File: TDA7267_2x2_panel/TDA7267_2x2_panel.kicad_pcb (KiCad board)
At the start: 2 copper layers, 90 x 84 mm, 72 parts, among them U1 TDA7267

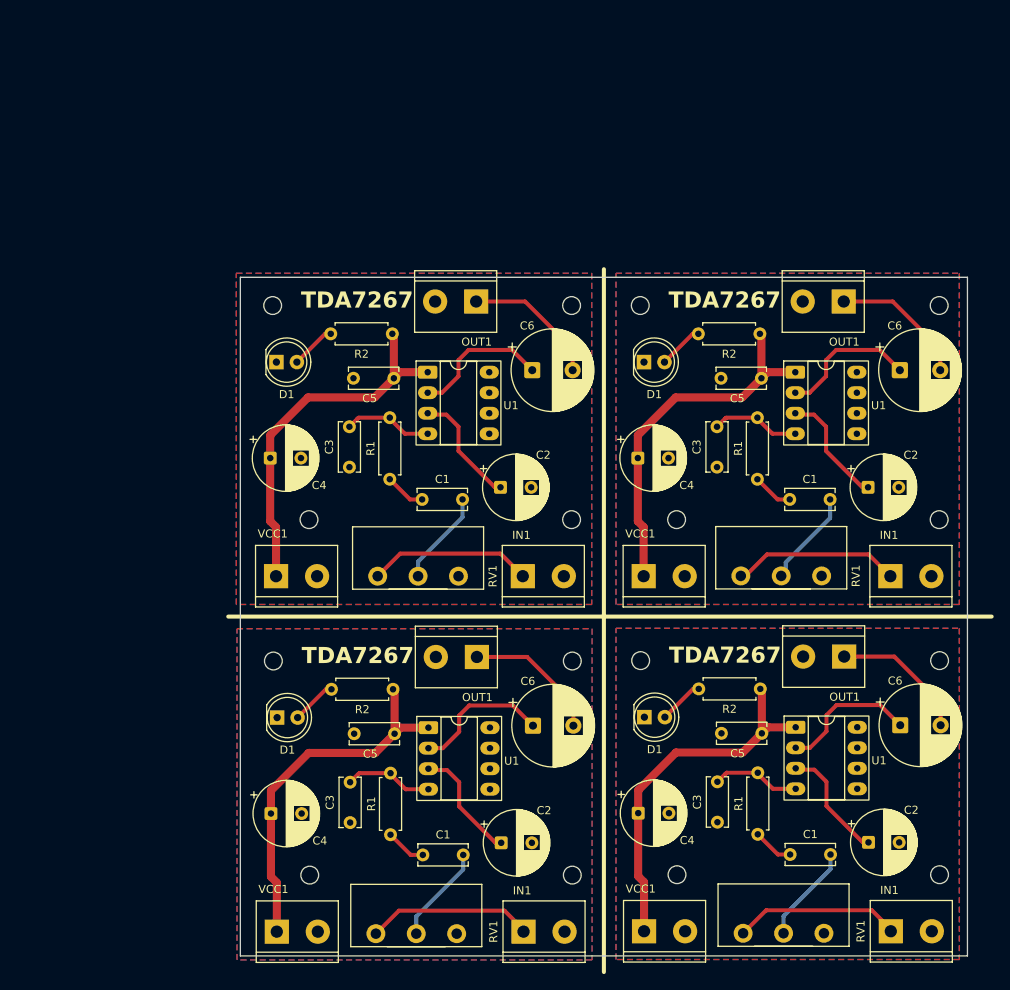
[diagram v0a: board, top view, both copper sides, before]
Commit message: Improvements
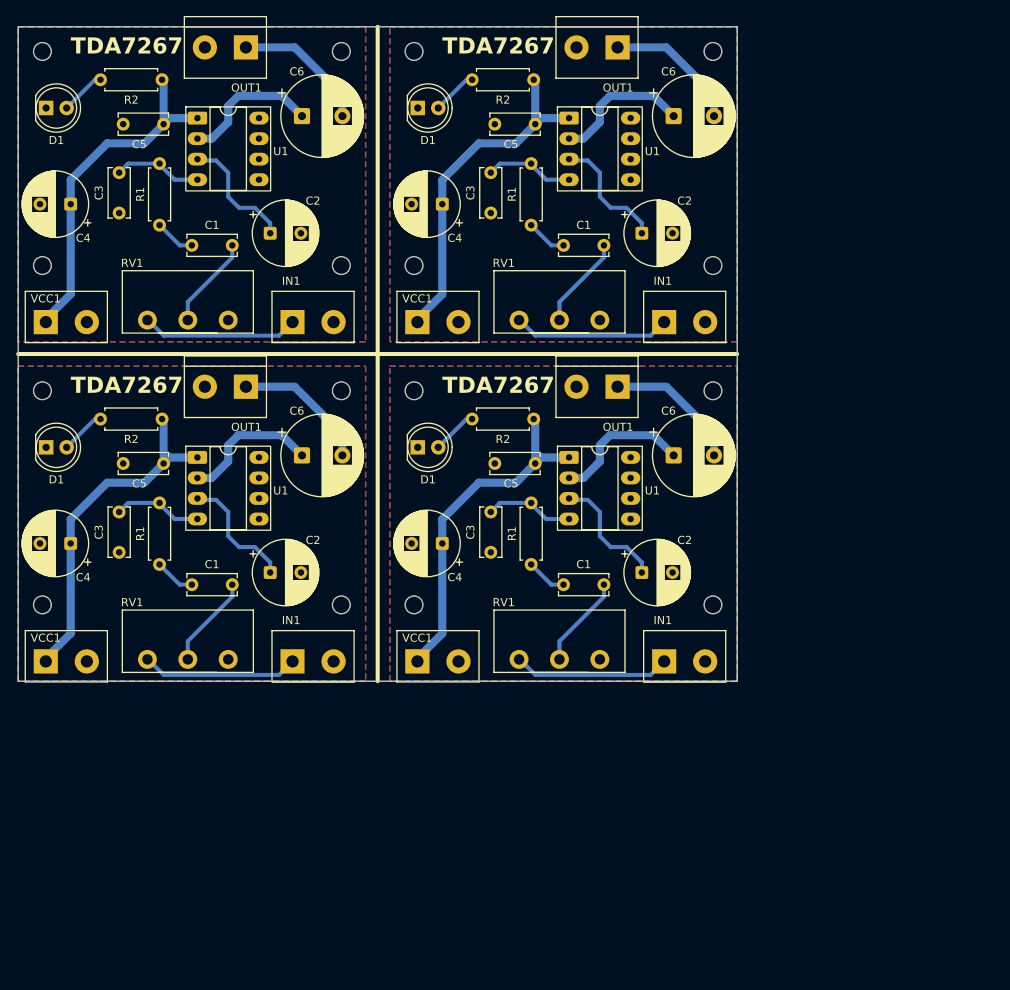
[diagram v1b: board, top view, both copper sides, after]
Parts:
- removed the C1 at (172.5, 87.5)
- removed the C1 at (127.1, 131.5)
- removed the C1 at (127.0, 87.5)
- removed the C1 at (172.6, 131.4)
- removed the C2 at (177.2, 129.9)
- removed the C2 at (131.7, 86.0)
- removed the C2 at (177.2, 86.0)
- removed the C2 at (131.8, 130.0)
- removed the C3 at (113.1, 127.5)
- removed the C3 at (158.5, 83.5)
- removed the C3 at (158.6, 127.5)
- removed the C3 at (113.0, 83.5)
- removed the C4 at (103.3, 126.4)
- removed the C4 at (148.8, 126.3)
- removed the C4 at (148.7, 82.4)
- removed the C4 at (103.2, 82.4)
- removed the C5 at (113.5, 72.5)
- removed the C5 at (159.0, 72.5)
- removed the C5 at (159.1, 116.5)
- removed the C5 at (113.6, 116.5)
- removed the C6 at (181.1, 71.5)
- removed the C6 at (135.7, 115.5)
- removed the C6 at (135.6, 71.5)
- removed the C6 at (181.2, 115.5)
- removed the D1 at (149.5, 70.5)
- removed the D1 at (104.0, 114.5)
- removed the D1 at (149.5, 114.5)
- removed the D1 at (104.0, 70.5)
- removed the H1 at (149.1, 107.5)
- removed the H1 at (103.6, 107.5)
- removed the H1 at (149.0, 63.5)
- removed the H1 at (103.5, 63.5)
- removed the H2 at (186.0, 63.5)
- removed the H2 at (140.6, 107.5)
- removed the H2 at (140.5, 63.5)
- removed the H2 at (186.1, 107.5)
- removed the H3 at (108.0, 90.0)
- removed the H3 at (153.5, 90.0)
- removed the H3 at (108.1, 134.0)
- removed the H3 at (153.6, 133.9)
- removed the H4 at (186.1, 133.9)
- removed the H4 at (186.0, 90.0)
- removed the H4 at (140.6, 134.0)
- removed the H4 at (140.5, 90.0)
- removed the IN1 at (134.5, 141.0)
- removed the IN1 at (180.0, 140.9)
- removed the IN1 at (180.0, 97.0)
- removed the IN1 at (134.5, 97.0)
- removed the OUT1 at (128.7, 63.0)
- removed the OUT1 at (174.2, 107.0)
- removed the OUT1 at (174.2, 63.0)
- removed the OUT1 at (128.8, 107.0)
- removed the R1 at (118.1, 129.0)
- removed the R1 at (163.6, 128.9)
- removed the R1 at (163.5, 85.0)
- removed the R1 at (118.0, 85.0)
- removed the R2 at (110.8, 111.0)
- removed the R2 at (156.2, 67.0)
- removed the R2 at (156.2, 111.0)
- removed the R2 at (110.7, 67.0)
- removed the RV1 at (116.3, 141.2)
- removed the RV1 at (116.5, 97.0)
- removed the RV1 at (161.4, 97.0)
- removed the RV1 at (161.7, 141.2)
- removed the U1 at (122.8, 115.8)
- removed the U1 at (168.2, 71.8)
- removed the U1 at (122.7, 71.8)
- removed the U1 at (168.2, 115.7)
- removed the VCC1 at (104.0, 141.0)
- removed the VCC1 at (149.4, 97.0)
- removed the VCC1 at (103.9, 97.0)
- removed the VCC1 at (149.5, 140.9)
- added C1: 1uF, Capacitor_THT:C_Disc_D6.0mm_W2.5mm_P5.00mm, F.Cu at (98.5, 56.0)
- added C1: 1uF, Capacitor_THT:C_Disc_D6.0mm_W2.5mm_P5.00mm, F.Cu at (144.5, 56.0)
- added C1: 1uF, Capacitor_THT:C_Disc_D6.0mm_W2.5mm_P5.00mm, F.Cu at (98.5, 98.0)
- added C1: 1uF, Capacitor_THT:C_Disc_D6.0mm_W2.5mm_P5.00mm, F.Cu at (144.5, 98.0)
- added C2: 47uF, Capacitor_THT:CP_Radial_D8.0mm_P3.80mm, F.Cu at (149.2, 96.5)
- added C2: 47uF, Capacitor_THT:CP_Radial_D8.0mm_P3.80mm, F.Cu at (149.2, 54.5)
- added C2: 47uF, Capacitor_THT:CP_Radial_D8.0mm_P3.80mm, F.Cu at (103.2, 54.5)
- added C2: 47uF, Capacitor_THT:CP_Radial_D8.0mm_P3.80mm, F.Cu at (103.2, 96.5)
- added C3: 470pF, Capacitor_THT:C_Disc_D6.0mm_W2.5mm_P5.00mm, F.Cu at (84.5, 94.0)
- added C3: 470pF, Capacitor_THT:C_Disc_D6.0mm_W2.5mm_P5.00mm, F.Cu at (84.5, 52.0)
- added C3: 470pF, Capacitor_THT:C_Disc_D6.0mm_W2.5mm_P5.00mm, F.Cu at (130.5, 52.0)
- added C3: 470pF, Capacitor_THT:C_Disc_D6.0mm_W2.5mm_P5.00mm, F.Cu at (130.5, 94.0)
- added C4: 100uF, Capacitor_THT:CP_Radial_D8.0mm_P3.80mm, F.Cu at (78.5, 51.0)
- added C4: 100uF, Capacitor_THT:CP_Radial_D8.0mm_P3.80mm, F.Cu at (78.5, 93.0)
- added C4: 100uF, Capacitor_THT:CP_Radial_D8.0mm_P3.80mm, F.Cu at (124.5, 51.0)
- added C4: 100uF, Capacitor_THT:CP_Radial_D8.0mm_P3.80mm, F.Cu at (124.5, 93.0)
- added C5: 100nF, Capacitor_THT:C_Disc_D6.0mm_W2.5mm_P5.00mm, F.Cu at (131.0, 83.0)
- added C5: 100nF, Capacitor_THT:C_Disc_D6.0mm_W2.5mm_P5.00mm, F.Cu at (85.0, 41.0)
- added C5: 100nF, Capacitor_THT:C_Disc_D6.0mm_W2.5mm_P5.00mm, F.Cu at (131.0, 41.0)
- added C5: 100nF, Capacitor_THT:C_Disc_D6.0mm_W2.5mm_P5.00mm, F.Cu at (85.0, 83.0)
- added C6: 1000uF, Capacitor_THT:CP_Radial_D10.0mm_P5.00mm, F.Cu at (153.1, 40.0)
- added C6: 1000uF, Capacitor_THT:CP_Radial_D10.0mm_P5.00mm, F.Cu at (107.1, 82.0)
- added C6: 1000uF, Capacitor_THT:CP_Radial_D10.0mm_P5.00mm, F.Cu at (153.1, 82.0)
- added C6: 1000uF, Capacitor_THT:CP_Radial_D10.0mm_P5.00mm, F.Cu at (107.1, 40.0)
- added D1: LED, LED_THT:LED_D5.0mm, F.Cu at (121.5, 39.0)
- added D1: LED, LED_THT:LED_D5.0mm, F.Cu at (121.5, 81.0)
- added D1: LED, LED_THT:LED_D5.0mm, F.Cu at (75.5, 39.0)
- added D1: LED, LED_THT:LED_D5.0mm, F.Cu at (75.5, 81.0)
- added H1: MountingHole, MountingHole:MountingHole_2.2mm_M2, F.Cu at (75.0, 74.0)
- added H1: MountingHole, MountingHole:MountingHole_2.2mm_M2, F.Cu at (121.0, 74.0)
- added H1: MountingHole, MountingHole:MountingHole_2.2mm_M2, F.Cu at (75.0, 32.0)
- added H1: MountingHole, MountingHole:MountingHole_2.2mm_M2, F.Cu at (121.0, 32.0)
- added H2: MountingHole, MountingHole:MountingHole_2.2mm_M2, F.Cu at (112.0, 74.0)
- added H2: MountingHole, MountingHole:MountingHole_2.2mm_M2, F.Cu at (158.0, 32.0)
- added H2: MountingHole, MountingHole:MountingHole_2.2mm_M2, F.Cu at (112.0, 32.0)
- added H2: MountingHole, MountingHole:MountingHole_2.2mm_M2, F.Cu at (158.0, 74.0)
- added H3: MountingHole, MountingHole:MountingHole_2.2mm_M2, F.Cu at (121.0, 58.5)
- added H3: MountingHole, MountingHole:MountingHole_2.2mm_M2, F.Cu at (75.0, 100.5)
- added H3: MountingHole, MountingHole:MountingHole_2.2mm_M2, F.Cu at (121.0, 100.5)
- added H3: MountingHole, MountingHole:MountingHole_2.2mm_M2, F.Cu at (75.0, 58.5)
- added H4: MountingHole, MountingHole:MountingHole_2.2mm_M2, F.Cu at (112.0, 100.5)
- added H4: MountingHole, MountingHole:MountingHole_2.2mm_M2, F.Cu at (158.0, 58.5)
- added H4: MountingHole, MountingHole:MountingHole_2.2mm_M2, F.Cu at (112.0, 58.5)
- added H4: MountingHole, MountingHole:MountingHole_2.2mm_M2, F.Cu at (158.0, 100.5)
- added IN1: Conn_01x02_Pin, TerminalBlock:TerminalBlock_bornier-2_P5.08mm, F.Cu at (106.0, 65.5)
- added IN1: Conn_01x02_Pin, TerminalBlock:TerminalBlock_bornier-2_P5.08mm, F.Cu at (152.0, 65.5)
- added IN1: Conn_01x02_Pin, TerminalBlock:TerminalBlock_bornier-2_P5.08mm, F.Cu at (106.0, 107.5)
- added IN1: Conn_01x02_Pin, TerminalBlock:TerminalBlock_bornier-2_P5.08mm, F.Cu at (152.0, 107.5)
- added OUT1: Conn_01x02_Pin, TerminalBlock:TerminalBlock_bornier-2_P5.08mm, F.Cu at (146.2, 73.5)
- added OUT1: Conn_01x02_Pin, TerminalBlock:TerminalBlock_bornier-2_P5.08mm, F.Cu at (100.2, 31.6)
- added OUT1: Conn_01x02_Pin, TerminalBlock:TerminalBlock_bornier-2_P5.08mm, F.Cu at (146.2, 31.6)
- added OUT1: Conn_01x02_Pin, TerminalBlock:TerminalBlock_bornier-2_P5.08mm, F.Cu at (100.2, 73.5)
- added R1: 1K, Resistor_THT:R_Axial_DIN0207_L6.3mm_D2.5mm_P7.62mm_Horizontal, F.Cu at (89.5, 53.5)
- added R1: 1K, Resistor_THT:R_Axial_DIN0207_L6.3mm_D2.5mm_P7.62mm_Horizontal, F.Cu at (135.5, 95.5)
- added R1: 1K, Resistor_THT:R_Axial_DIN0207_L6.3mm_D2.5mm_P7.62mm_Horizontal, F.Cu at (89.5, 95.5)
- added R1: 1K, Resistor_THT:R_Axial_DIN0207_L6.3mm_D2.5mm_P7.62mm_Horizontal, F.Cu at (135.5, 53.5)
- added R2: 1K, Resistor_THT:R_Axial_DIN0207_L6.3mm_D2.5mm_P7.62mm_Horizontal, F.Cu at (82.2, 77.5)
- added R2: 1K, Resistor_THT:R_Axial_DIN0207_L6.3mm_D2.5mm_P7.62mm_Horizontal, F.Cu at (128.2, 77.5)
- added R2: 1K, Resistor_THT:R_Axial_DIN0207_L6.3mm_D2.5mm_P7.62mm_Horizontal, F.Cu at (128.2, 35.5)
- added R2: 1K, Resistor_THT:R_Axial_DIN0207_L6.3mm_D2.5mm_P7.62mm_Horizontal, F.Cu at (82.2, 35.5)
- added RV1: R_Potentiometer, Potentiometer_THT:Potentiometer_Piher_T-16H_Single_Horizontal, F.Cu at (88.0, 65.3)
- added RV1: R_Potentiometer, Potentiometer_THT:Potentiometer_Piher_T-16H_Single_Horizontal, F.Cu at (88.0, 107.3)
- added RV1: R_Potentiometer, Potentiometer_THT:Potentiometer_Piher_T-16H_Single_Horizontal, F.Cu at (134.0, 107.3)
- added RV1: R_Potentiometer, Potentiometer_THT:Potentiometer_Piher_T-16H_Single_Horizontal, F.Cu at (134.0, 65.3)
- added U1: TDA7267, Package_DIP:DIP-8_W7.62mm_Socket_LongPads, F.Cu at (140.2, 82.3)
- added U1: TDA7267, Package_DIP:DIP-8_W7.62mm_Socket_LongPads, F.Cu at (94.2, 82.3)
- added U1: TDA7267, Package_DIP:DIP-8_W7.62mm_Socket_LongPads, F.Cu at (94.2, 40.3)
- added U1: TDA7267, Package_DIP:DIP-8_W7.62mm_Socket_LongPads, F.Cu at (140.2, 40.3)
- added VCC1: Conn_01x02_Pin, TerminalBlock:TerminalBlock_bornier-2_P5.08mm, F.Cu at (121.4, 107.5)
- added VCC1: Conn_01x02_Pin, TerminalBlock:TerminalBlock_bornier-2_P5.08mm, F.Cu at (121.4, 65.5)
- added VCC1: Conn_01x02_Pin, TerminalBlock:TerminalBlock_bornier-2_P5.08mm, F.Cu at (75.4, 107.5)
- added VCC1: Conn_01x02_Pin, TerminalBlock:TerminalBlock_bornier-2_P5.08mm, F.Cu at (75.4, 65.5)
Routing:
- net Net-(U1-V+): track 184.2 -> 173.3 mm
- net Net-(IN1-Pin_1): track 81.9 -> 78.0 mm
- net Net-(U1-SRV): track 58.3 -> 61.2 mm
- net Net-(C1-Pad1): track 47.9 -> 45.7 mm
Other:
- board size 90 x 84 mm -> 89 x 81 mm
